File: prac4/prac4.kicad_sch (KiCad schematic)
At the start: 5 parts, among them J1 Screw_Terminal_01x04

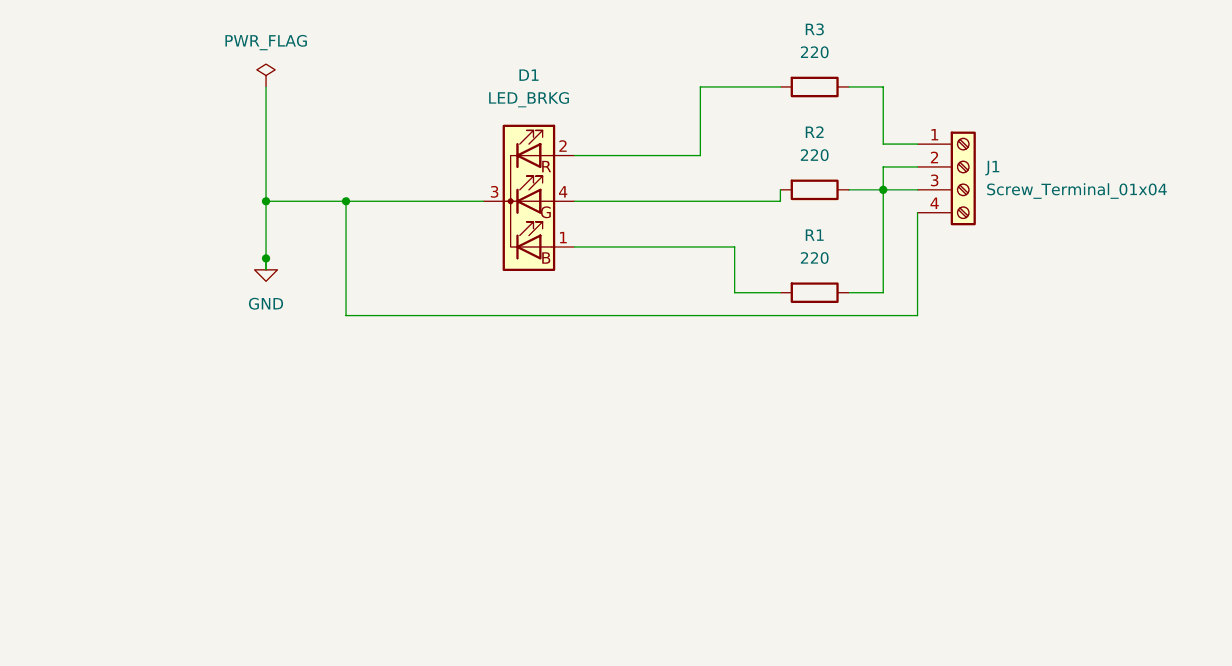
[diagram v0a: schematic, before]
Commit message: prac 4 2do parcial
prac 4 2do parcial
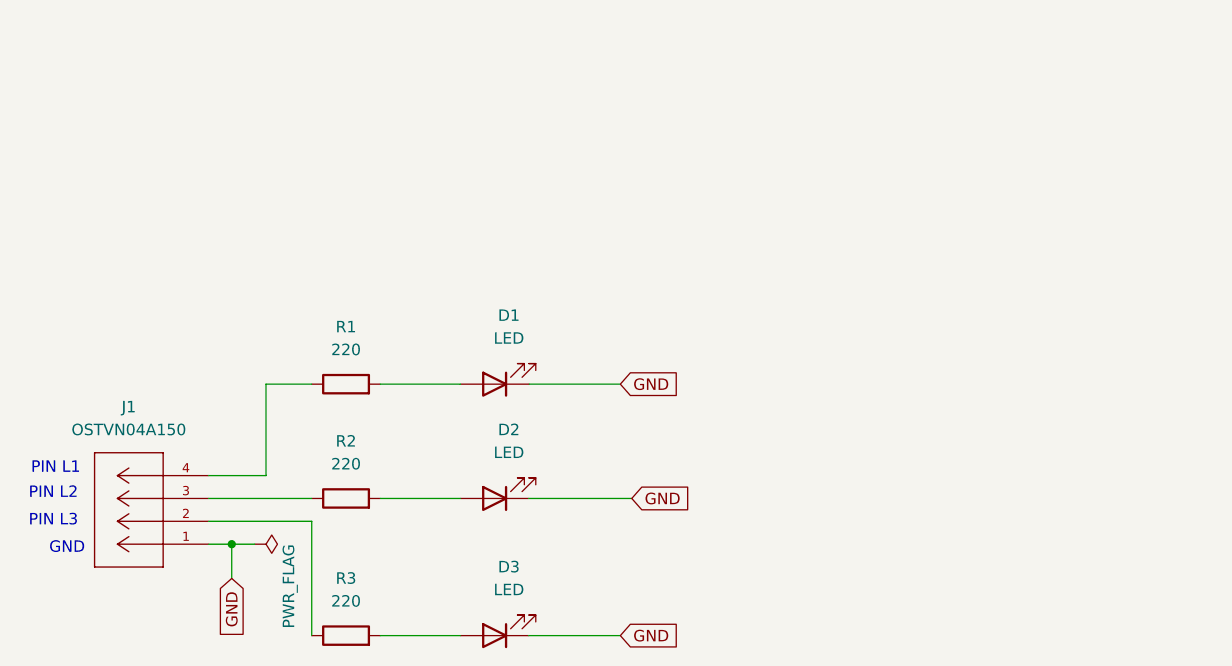
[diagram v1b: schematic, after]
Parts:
- removed D1: LED_BRKG, LED_SMD:LED_RGB_1210, symbol Device:LED_BRKG
- removed J1: Screw_Terminal_01x04, TerminalBlock_Phoenix:TerminalBlock_Phoenix_MKDS-1,5-4-5.08_1x04_P5.08mm_Horizontal, symbol Connector:Screw_Terminal_01x04
- added D1, D2, D3: LED, LED_LTL-4233_LTO:LED_LTL-4233_LTO, symbol Device:LED
- added J1: OSTVN04A150, TerminalBlock_OSTVN04A150:TerminalBlock_OSTVN04A150, symbol TerminalBlock_OSTVN04A150:OSTVN04A150
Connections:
- net GND: now also D1.1 (K), D2.1 (K), D3.1 (K), J1.1
- net at R2.1: now also J1.3; no longer R1.1
- net at R1.2: now also D1.2 (A)
- net at R3.1: now also J1.2
- net at R3.2: now also D3.2 (A)
- net at R2.2: now also D2.2 (A)
- new net: J1.4, R1.1
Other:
- note added: "GND"
- note added: "PIN L1"
- note added: "PIN L2"
- note added: "PIN L3"
